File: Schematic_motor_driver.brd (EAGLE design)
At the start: 49.8 x 49.8 mm, 29 parts, among them Q2 IRF540, Q3 IRF540, Q4 IRF540, Q5 IRF540, U1 IR2104PBF, U2 IR2104PBF

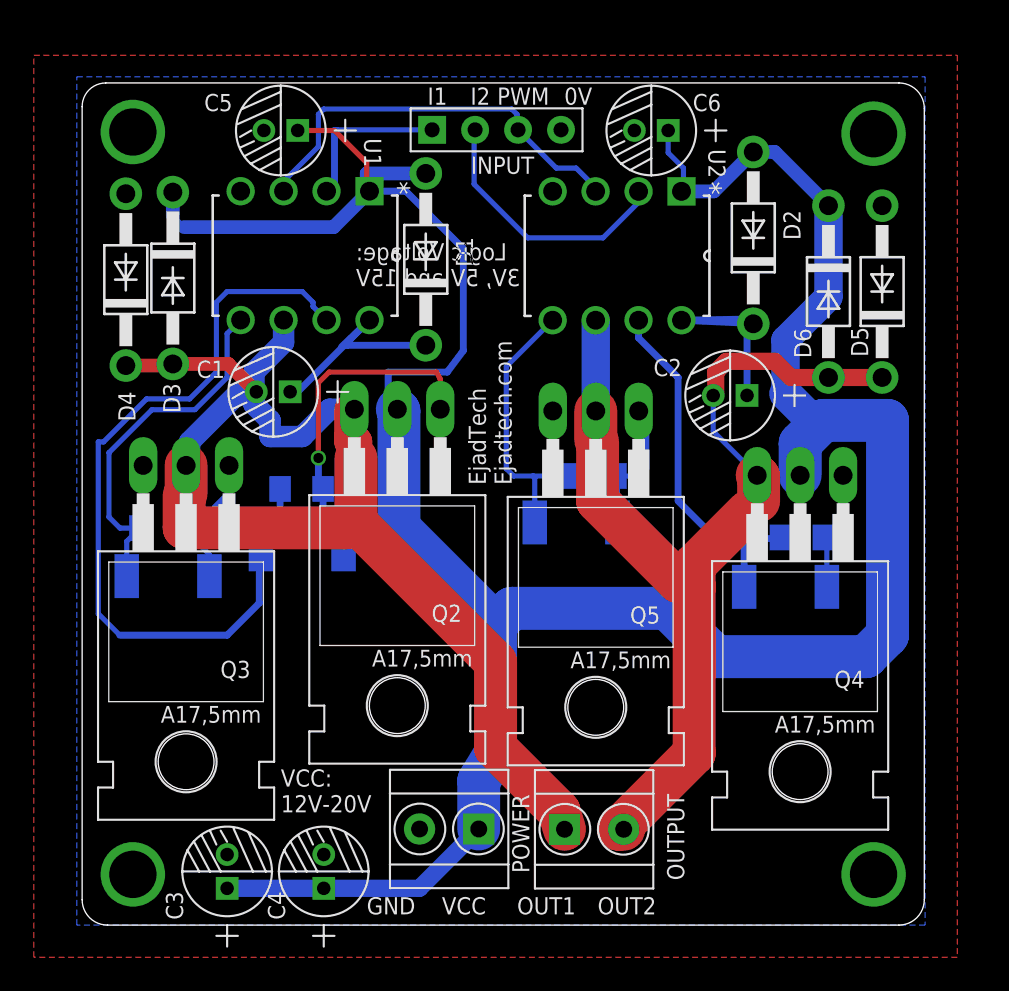
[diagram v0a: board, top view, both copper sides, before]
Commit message: adding latest files to git repo
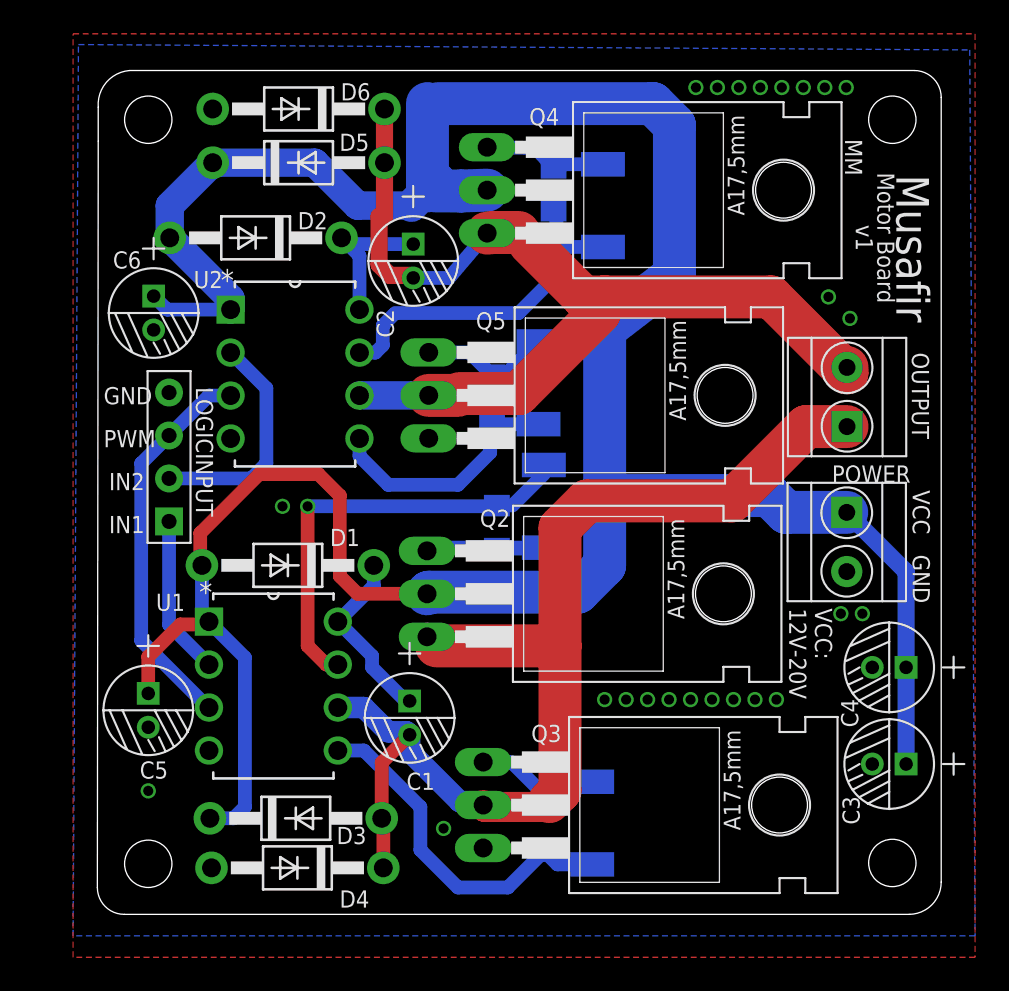
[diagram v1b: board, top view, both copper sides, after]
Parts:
- removed INPUT: 4p-2.54, Seeed-Connector -2016:H4-2.54
- added LOGICINPUT: 4p-2.54, Seeed-Connector -2016:H4-2.54
- moved C3 39.7 mm to (47.7, 9.53), turned to 180 degrees
- moved D4 36.2 mm to (12.7, 3.38), turned to 180 degrees
- moved D6 36.2 mm to (12.8, 48.3), turned to 180 degrees
- moved C4 35.5 mm to (47.7, 15.2), turned to 180 degrees
- moved C5 35.2 mm to (3.91, 12.7), turned to 270 degrees
- moved D3 32.8 mm to (12.6, 6.32), turned to 0 degrees
- moved D5 32.2 mm to (12.8, 45.1), turned to 0 degrees
- moved C6 31.3 mm to (4.23, 36.2), turned to 270 degrees
- moved OUTPUT 29.6 mm to (45.2, 31.2), turned to 90 degrees
- moved D2 29.4 mm to (10.3, 40.6), turned to 180 degrees
- moved D8 29.0 mm to (30.2, 6.03), turned to 90 degrees
- moved POWER 29.0 mm to (45.2, 22.7), turned to 270 degrees
- moved R2 28.8 mm to (27.3, 5.64), turned to 90 degrees
- moved Q3 27.6 mm to (30.1, 7.10), turned to 270 degrees
- moved Q4 26.2 mm to (30.3, 43.5), turned to 270 degrees
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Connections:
- net GND: now also LOGICINPUT.4; no longer INPUT.4
- net IN1: now also LOGICINPUT.1; no longer INPUT.1
- net IN2: now also LOGICINPUT.2; no longer INPUT.2
- net PWM: now also LOGICINPUT.3; no longer INPUT.3
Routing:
- net N$7: track 48.7 -> 25.8 mm, vias 0 -> 1
- net N$6: track 20.2 -> 9.79 mm, vias 1 -> 0
- net POWER: track 165.4 -> 172.9 mm
- net VS1: track 73.8 -> 68.2 mm
- net N$4: track 13.5 -> 9.08 mm
- net IN2: track 16.9 -> 13.6 mm
- net N$2: track 13.6 -> 10.8 mm
- net PWM: track 24.7 -> 23.1 mm
- net N$10: track 16.8 -> 15.2 mm
- net VS2: track 61.0 -> 59.8 mm
- net N$8: track 21.9 -> 21.1 mm
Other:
- board size 49.8 x 49.8 mm -> 49.9 x 49.9 mm
- board text added: "IN1"
- board text added: "IN2"
- board text added: "MM"
- board text added: "Motor Board"
- board text added: "Musafir"
- board text added: "ejaadtech.com"
- board text added: "v1"
- board text removed: "0V"
- board text removed: "EjadTech Ejadtech.com"
- board text removed: "I1"
- board text removed: "I2"
- board text removed: "Logic Voltage: 3V, 5V and 15V"
- board text removed: "OUT1"
- board text removed: "OUT2"
